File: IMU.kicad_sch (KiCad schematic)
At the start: 5 parts, among them J3 5033981892, U1 ICM-42688-P

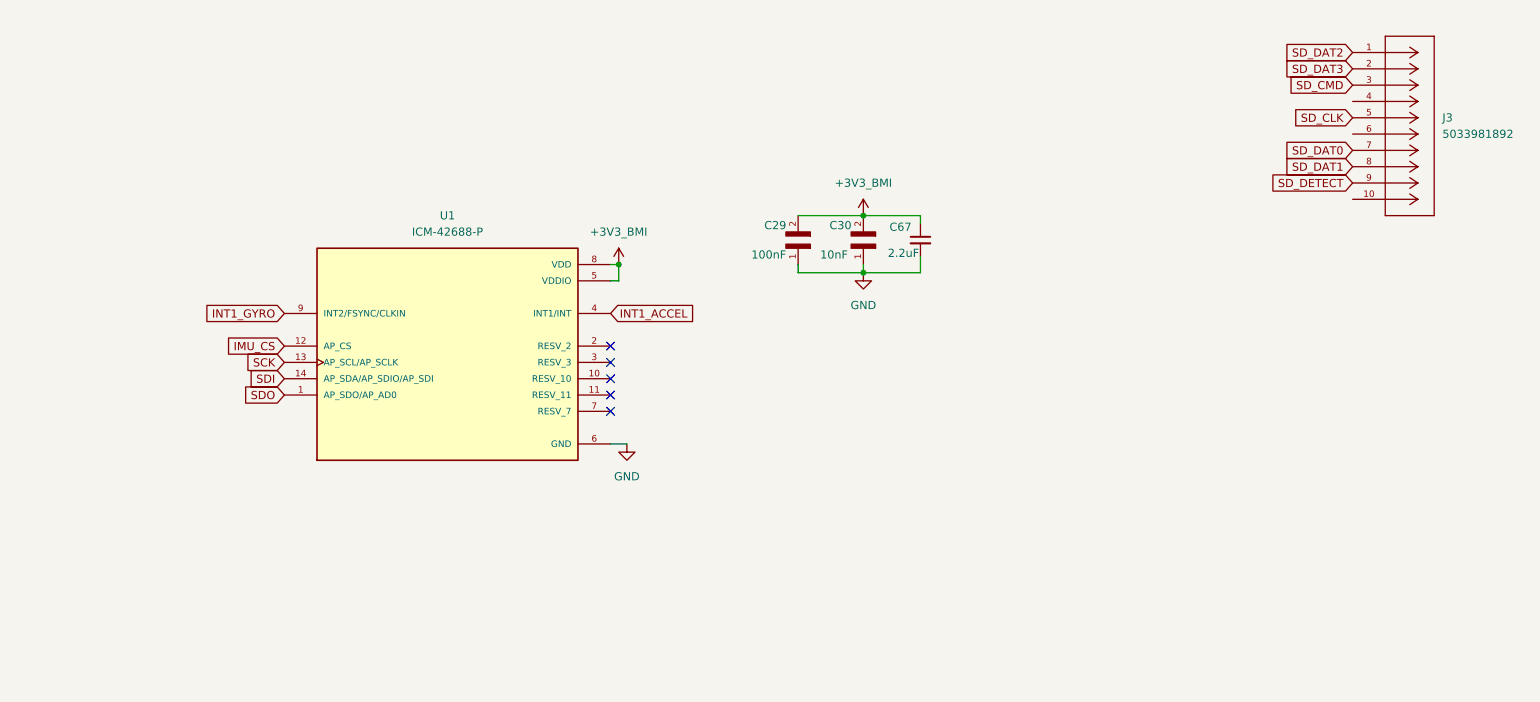
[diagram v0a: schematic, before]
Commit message: new can
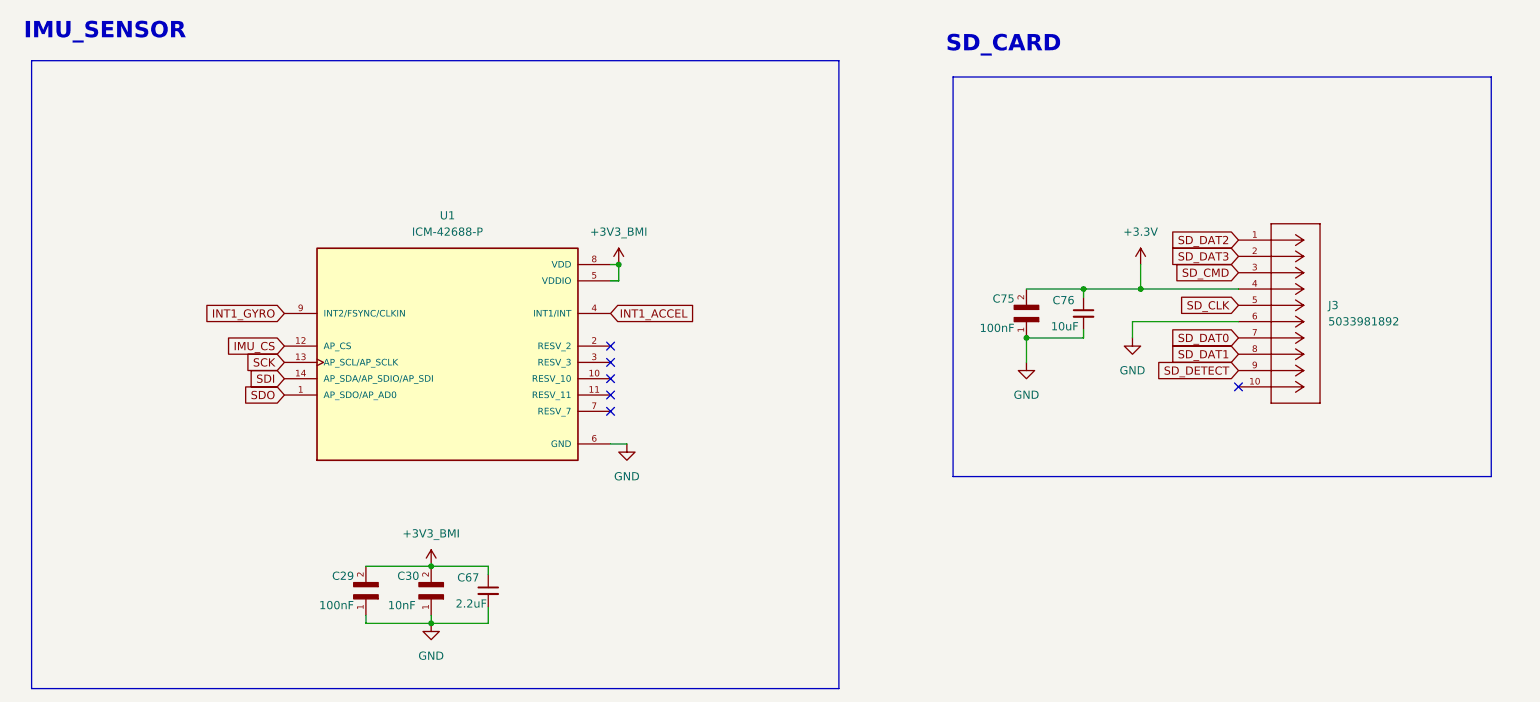
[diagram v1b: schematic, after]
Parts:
- added C75: 100nF, C0402C104K4RAC:CAPC1005X55N, symbol C0402C104K4RAC:C0402C104K4RAC
- added C76: 10uF, Capacitor_SMD:C_0805_2012Metric, symbol Device:C_Small
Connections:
- net GND: now also J3.6, C75.1, C76.2
- net +3.3V: now reaches J3.4
- net +3.3V: now also C75.2, C76.1
- no-connect marks 5 -> 6
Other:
- note added: "IMU_SENSOR"
- note added: "SD_CARD"
- moved on the sheet: C29, C30, C67, J3

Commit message: schamtic Update
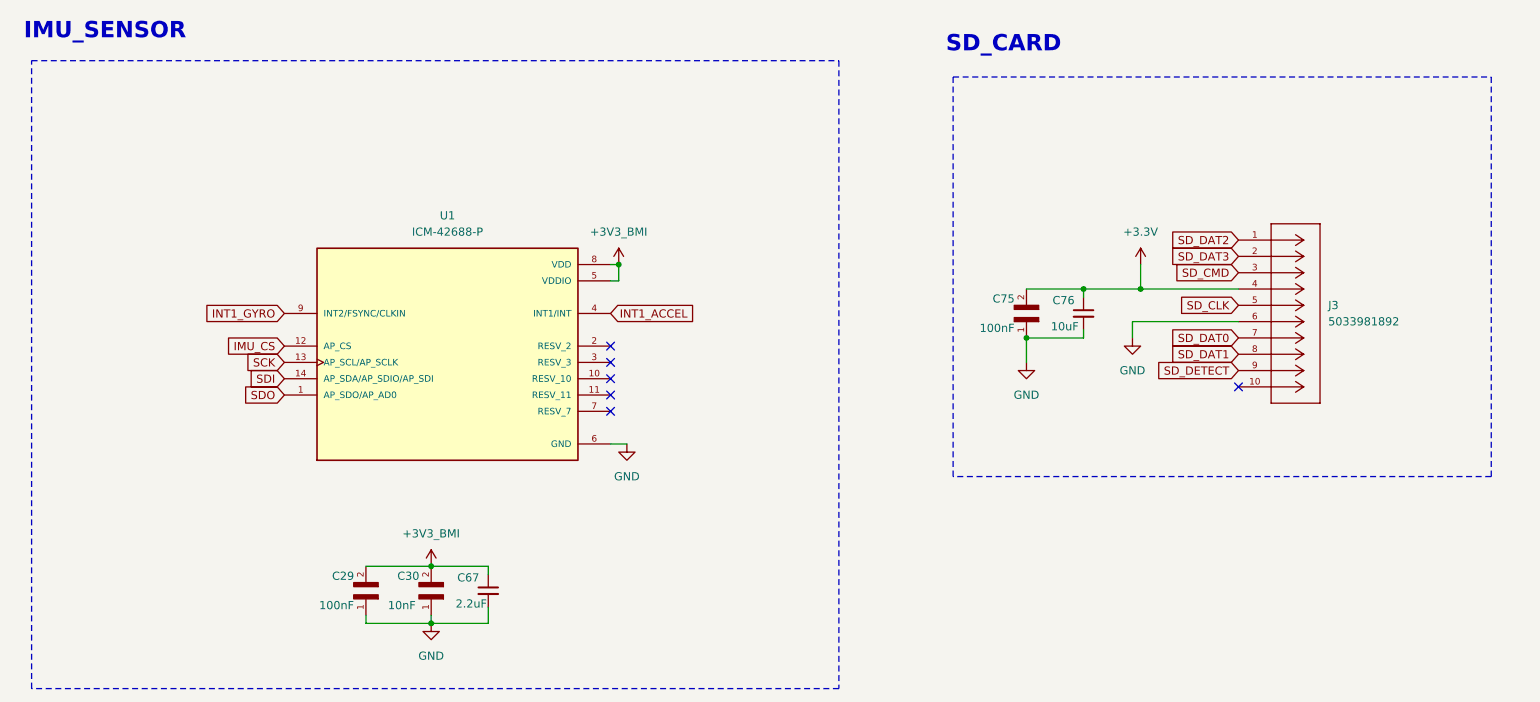
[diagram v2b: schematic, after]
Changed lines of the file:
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@@
 		(end 163.83 162.56)
 		(stroke
-			(width 0)
-			(type default)
+			(width 0.0508)
+			(type dash)
+			(color 0 0 0 1)
 		)
 		(fill
@@
 		(end 265.43 129.54)
 		(stroke
-			(width 0)
-			(type default)
+			(width 0.0508)
+			(type dash)
+			(color 0 0 0 1)
 		)
 		(fill
